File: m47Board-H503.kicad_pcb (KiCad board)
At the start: 2 copper layers, 42 parts, among them J1 USB_C_Receptacle_USB2.0_14P, J3 Conn_01x15_Pin, J4 Conn_01x10_Pin, J5 Conn_01x15_Pin, SW1 SW_Push, SW2 SW_Push, SW3 SW_Push, U1 AP2114H-3.3TRG1, U2 STM32H503CBTx, U3 USBLC6-2SC6, Y1 CX3225FB16000F0FZZH1 16MHz, Y2 ABS07-32.768KHZ-T

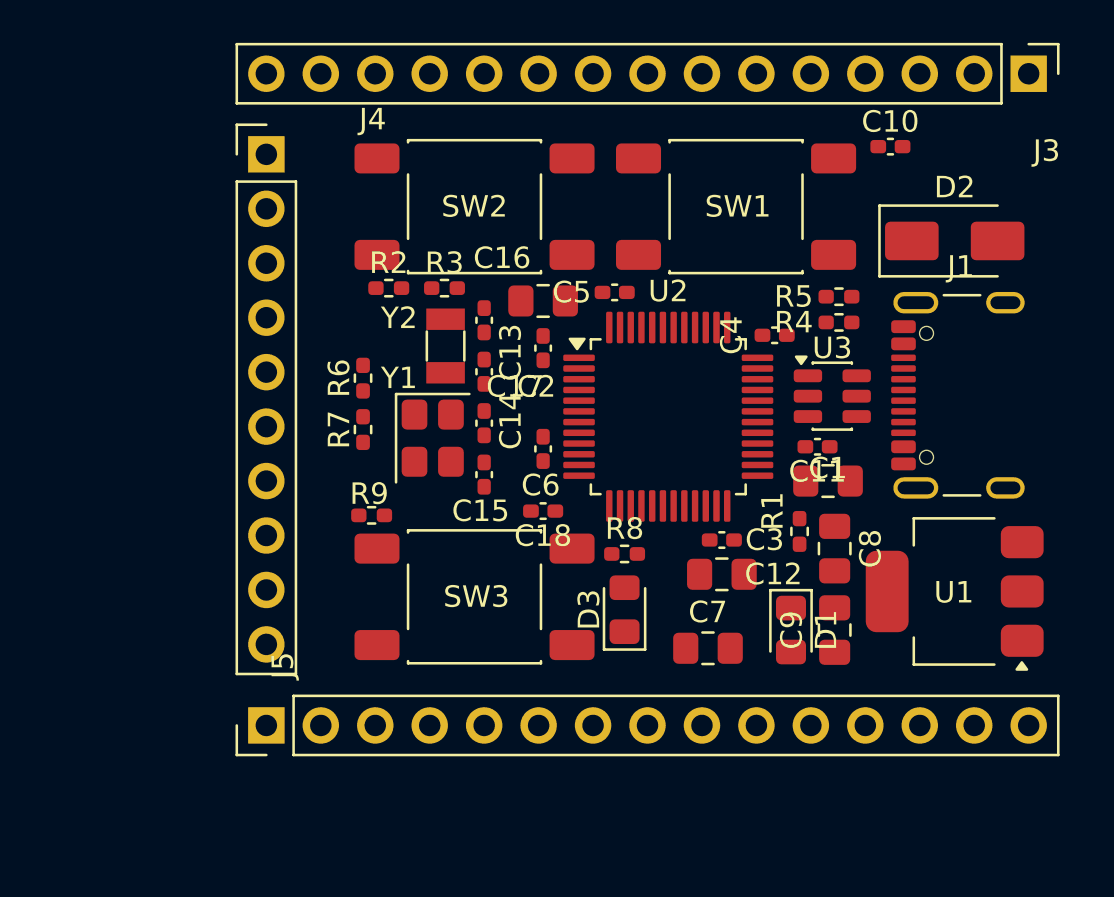
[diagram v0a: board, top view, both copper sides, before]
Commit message: Update PCB layout
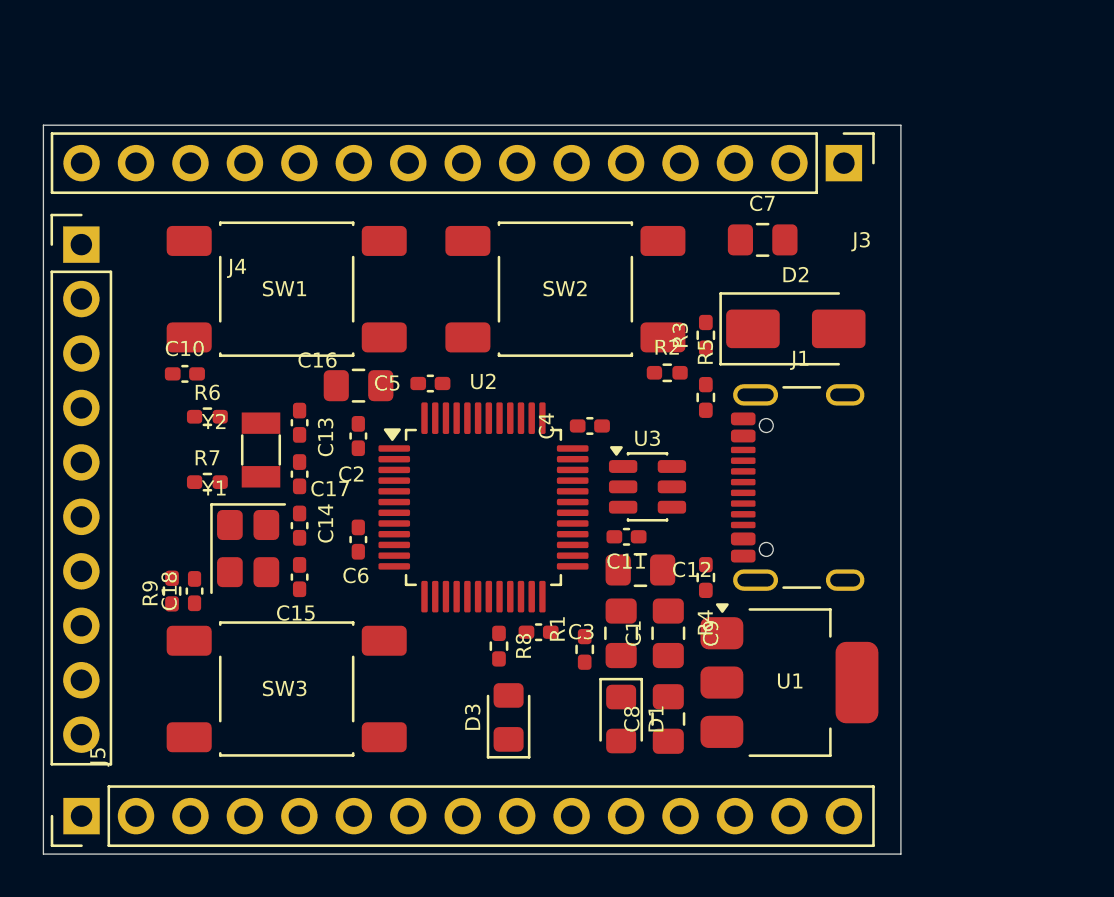
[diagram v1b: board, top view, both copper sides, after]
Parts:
- moved C10 34.6 mm to (126.6, 97.6)
- moved SW1 21.3 mm to (131.3, 93.7), turned to 0 degrees
- moved C7 19.2 mm to (153.6, 91.3)
- moved C18 16.7 mm to (127.0, 107.7), turned to 90 degrees
- moved R2 13.6 mm to (149.1, 97.5)
- moved R4 13.4 mm to (150.9, 107.1), turned to -90 degrees
- moved R3 12.4 mm to (150.9, 95.8), turned to 90 degrees
- moved C1 12.0 mm to (146.9, 109.7), turned to -90 degrees
- moved R1 11.4 mm to (145.2, 110.5)
- moved C8 11.1 mm to (149.2, 113.7), turned to 90 degrees
- moved Y1 10.0 mm to (129.6, 105.8)
- moved R9 9.96 mm to (126.0, 107.7), turned to -90 degrees
- moved Y2 9.88 mm to (130.2, 101.2)
- moved C11 9.85 mm to (147.2, 105.2)
- moved C14 9.85 mm to (131.9, 104.7)
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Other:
- board outline added: 40 x 34 mm

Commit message: Update PCB layout
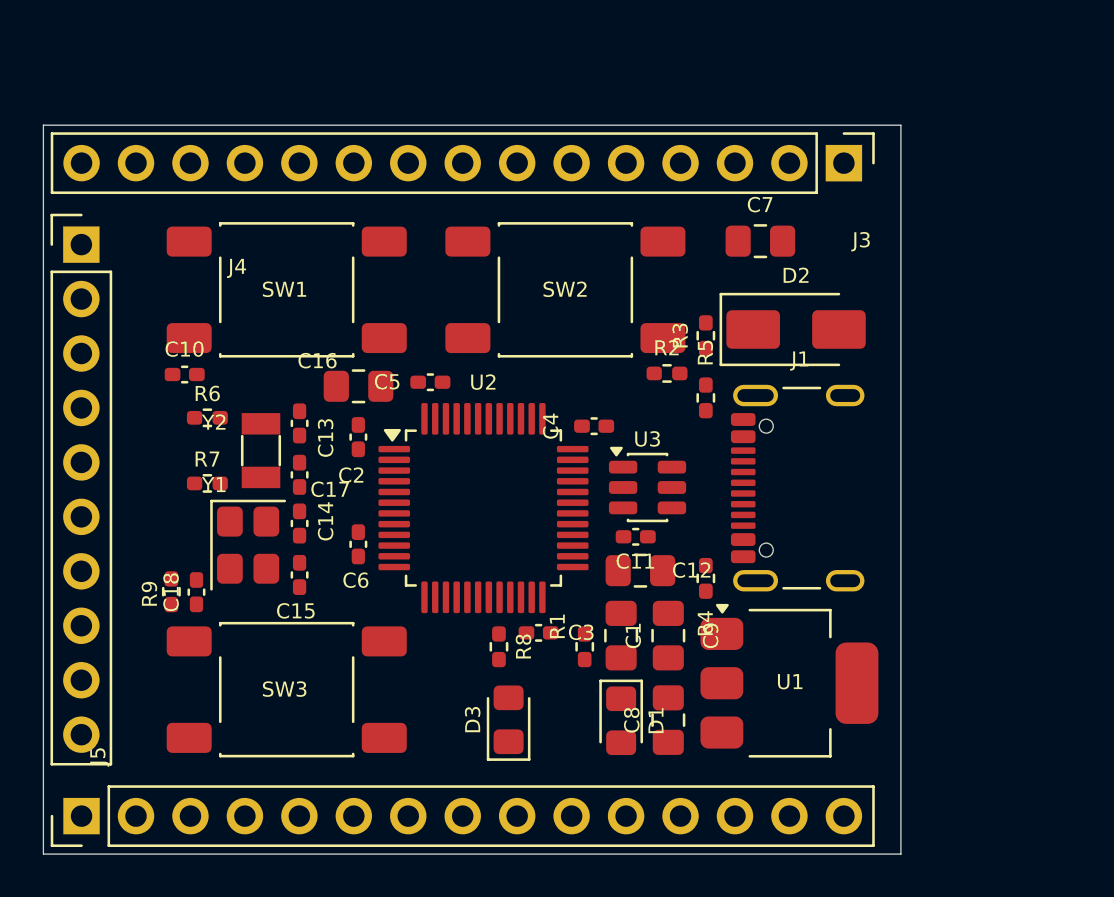
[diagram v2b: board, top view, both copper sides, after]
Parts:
- moved C11 0.43 mm to (147.6, 105.2)
- moved C6 0.22 mm to (134.7, 105.5)
- moved C4 0.20 mm to (145.7, 100.0)
- moved Y1 0.16 mm to (129.6, 105.6)
- moved R1 0.12 mm to (145.2, 110.3)
- moved C7 0.12 mm to (153.4, 91.4)
- moved C1 0.11 mm to (146.9, 109.8)
- moved C9 0.11 mm to (149.2, 109.8)
- moved D3 0.11 mm to (141.7, 113.7)
- moved C18 0.10 mm to (127.1, 107.8)
- moved C14 0.10 mm to (131.9, 104.6)
- moved C15 0.10 mm to (131.9, 107.0)
- moved D1 0.08 mm to (146.9, 113.8)
- moved C5 0.06 mm to (138.1, 98.0)
- moved R7 0.06 mm to (127.7, 102.7)
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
